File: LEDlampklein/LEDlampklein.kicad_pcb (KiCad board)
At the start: 2 copper layers, 4.8 x 17 mm, 6 parts

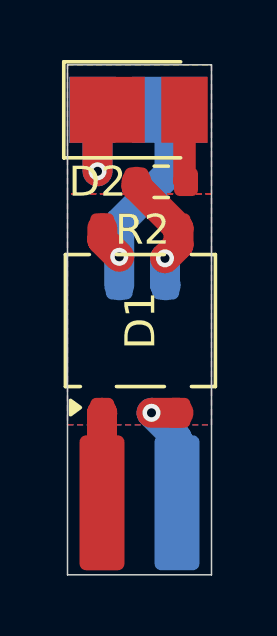
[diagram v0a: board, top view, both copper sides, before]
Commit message: erc lamp
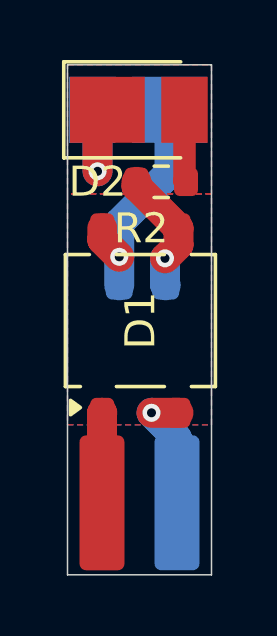
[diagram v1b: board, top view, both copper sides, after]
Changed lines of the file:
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@@
 			(psa4output no)
 			(plot_black_and_white yes)
-			(plotinvisibletext no)
 			(sketchpadsonfab no)
 			(plotpadnumbers no)
@@
 			)
 		)
-		(property "Datasheet" ""
+		(property "Datasheet" "~"
 			(at 0 0 0)
 			(unlocked yes)
@@
 			)
 		)
-		(property "Datasheet" ""
+		(property "Datasheet" "~"
 			(at 0 0 0)
 			(unlocked yes)
@@
 		)
 		(embedded_fonts no)
-		(model "${KICAD9_3DMODEL_DIR}/LED_SMD.3dshapes/LED_PLCC_2835.wrl"
+		(model "${KICAD9_3DMODEL_DIR}/LED_SMD.3dshapes/LED_PLCC_2835.step"
 			(offset
 				(xyz 0 0 0)
@@
 		(layer "F.Cu")
 		(at 93.125 66.9)
-		(descr "Resistor SMD 0603 (1608 Metric), square (rectangular) end terminal, IPC_7351 nominal, (Body size source: IPC-SM-782 page 72, https://www.pcb-3d.com/wordpress/wp-content/uploads/ipc-sm-782a_amendment_1_and_2.pdf), generated with kicad-footprint-generator")
+		(descr "Resistor SMD 0603 (1608 Metric), square (rectangular) end terminal, IPC-7351 nominal, (Body size source: IPC-SM-782 page 72, https://www.pcb-3d.com/wordpress/wp-content/uploads/ipc-sm-782a_amendment_1_and_2.pdf), generated with kicad-footprint-generator")
 		(tags "resistor")
 		(property "Reference" "R2"
-			(at -0.625 1.6 0)
-			(layer "F.SilkS")
-			(effects
-				(font
-					(size 1 1)
-					(thickness 0.15)
+			(at -0.669 1.553 0)
+			(layer "F.SilkS")
+			(effects
+				(font
+					(size 1 1)
+					(thickness 0.1)
 				)
 			)
@@
 			)
 		)
-		(property "Datasheet" ""
+		(property "Datasheet" "~"
 			(at 0 0 0)
 			(unlocked yes)
@@
 			(layer "F.SilkS")
 		)
-		(fp_line
+		(fp_rect
 			(start -1.48 -0.73)
-			(end 1.48 -0.73)
-			(stroke
-				(width 0.05)
-				(type solid)
-			)
+			(end 1.48 0.73)
+			(stroke
+				(width 0.05)
+				(type solid)
+			)
+			(fill no)
 			(layer "F.CrtYd")
 		)
-		(fp_line
-			(start -1.48 0.73)
-			(end -1.48 -0.73)
-			(stroke
-				(width 0.05)
-				(type solid)
-			)
-			(layer "F.CrtYd")
-		)
-		(fp_line
-			(start 1.48 -0.73)
-			(end 1.48 0.73)
-			(stroke
-				(width 0.05)
-				(type solid)
-			)
-			(layer "F.CrtYd")
-		)
-		(fp_line
-			(start 1.48 0.73)
-			(end -1.48 0.73)
-			(stroke
-				(width 0.05)
-				(type solid)
-			)
-			(layer "F.CrtYd")
-		)
-		(fp_line
+		(fp_rect
 			(start -0.8 -0.4125)
-			(end 0.8 -0.4125)
-			(stroke
-				(width 0.1)
-				(type solid)
-			)
-			(layer "F.Fab")
-		)
-		(fp_line
-			(start -0.8 0.4125)
-			(end -0.8 -0.4125)
-			(stroke
-				(width 0.1)
-				(type solid)
-			)
-			(layer "F.Fab")
-		)
-		(fp_line
-			(start 0.8 -0.4125)
 			(end 0.8 0.4125)
 			(stroke
@@
 				(type solid)
 			)
-			(layer "F.Fab")
-		)
-		(fp_line
-			(start 0.8 0.4125)
-			(end -0.8 0.4125)
-			(stroke
-				(width 0.1)
-				(type solid)
-			)
+			(fill no)
 			(layer "F.Fab")
 		)
@@
 		)
 		(embedded_fonts no)
-		(model "${KICAD9_3DMODEL_DIR}/Resistor_SMD.3dshapes/R_0603_1608Metric.wrl"
+		(model "${KICAD9_3DMODEL_DIR}/Resistor_SMD.3dshapes/R_0603_1608Metric.step"
 			(offset
 				(xyz 0 0 0)
@@
 		)
 		(embedded_fonts no)
-		(model "${KICAD9_3DMODEL_DIR}/Package_TO_SOT_SMD.3dshapes/TO-269AA.wrl"
+		(model "${KICAD9_3DMODEL_DIR}/Package_TO_SOT_SMD.3dshapes/TO-269AA.step"
 			(offset
 				(xyz 0 0 0)
@@
 			)
 		)
-		(property "Datasheet" ""
+		(property "Datasheet" "~"
 			(at 0 0 0)
 			(unlocked yes)
@@
 		)
 		(embedded_fonts no)
-		(model "${KICAD9_3DMODEL_DIR}/LED_SMD.3dshapes/LED_PLCC_2835.wrl"
+		(model "${KICAD9_3DMODEL_DIR}/LED_SMD.3dshapes/LED_PLCC_2835.step"
 			(offset
 				(xyz 0 0 0)
@@
 		(layer "B.Cu")
 		(at 92.5 70.35 180)
-		(descr "Capacitor SMD 0603 (1608 Metric), square (rectangular) end terminal, IPC_7351 nominal, (Body size source: IPC-SM-782 page 76, https://www.pcb-3d.com/wordpress/wp-content/uploads/ipc-sm-782a_amendment_1_and_2.pdf), generated with kicad-footprint-generator")
+		(descr "Capacitor SMD 0603 (1608 Metric), square (rectangular) end terminal, IPC-7351 nominal, (Body size source: IPC-SM-782 page 76, https://www.pcb-3d.com/wordpress/wp-content/uploads/ipc-sm-782a_amendment_1_and_2.pdf), generated with kicad-footprint-generator")
 		(tags "capacitor")
 		(property "Reference" "C4"
@@
 			)
 		)
-		(property "Datasheet" ""
+		(property "Datasheet" "~"
 			(at 0 0 0)
 			(unlocked yes)
@@
 			(layer "B.SilkS")
 		)
-		(fp_line
-			(start 1.48 0.73)
+		(fp_rect
+			(start -1.48 0.73)
 			(end 1.48 -0.73)
 			(stroke
@@
 				(type solid)
 			)
+			(fill no)
 			(layer "B.CrtYd")
 		)
-		(fp_line
-			(start 1.48 -0.73)
-			(end -1.48 -0.73)
-			(stroke
-				(width 0.05)
-				(type solid)
-			)
-			(layer "B.CrtYd")
-		)
-		(fp_line
-			(start -1.48 0.73)
-			(end 1.48 0.73)
-			(stroke
-				(width 0.05)
-				(type solid)
-			)
-			(layer "B.CrtYd")
-		)
-		(fp_line
-			(start -1.48 -0.73)
-			(end -1.48 0.73)
-			(stroke
-				(width 0.05)
-				(type solid)
-			)
-			(layer "B.CrtYd")
-		)
-		(fp_line
-			(start 0.8 0.4)
+		(fp_rect
+			(start -0.8 0.4)
 			(end 0.8 -0.4)
 			(stroke
@@
 				(type solid)
 			)
-			(layer "B.Fab")
-		)
-		(fp_line
-			(start 0.8 -0.4)
-			(end -0.8 -0.4)
-			(stroke
-				(width 0.1)
-				(type solid)
-			)
-			(layer "B.Fab")
-		)
-		(fp_line
-			(start -0.8 0.4)
-			(end 0.8 0.4)
-			(stroke
-				(width 0.1)
-				(type solid)
-			)
-			(layer "B.Fab")
-		)
-		(fp_line
-			(start -0.8 -0.4)
-			(end -0.8 0.4)
-			(stroke
-				(width 0.1)
-				(type solid)
-			)
+			(fill no)
 			(layer "B.Fab")
 		)
@@
 		)
 		(embedded_fonts no)
-		(model "${KICAD9_3DMODEL_DIR}/Capacitor_SMD.3dshapes/C_0603_1608Metric.wrl"
+		(model "${KICAD9_3DMODEL_DIR}/Capacitor_SMD.3dshapes/C_0603_1608Metric.step"
 			(offset
 				(xyz 0 0 0)
